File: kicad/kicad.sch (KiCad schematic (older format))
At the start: 40 parts

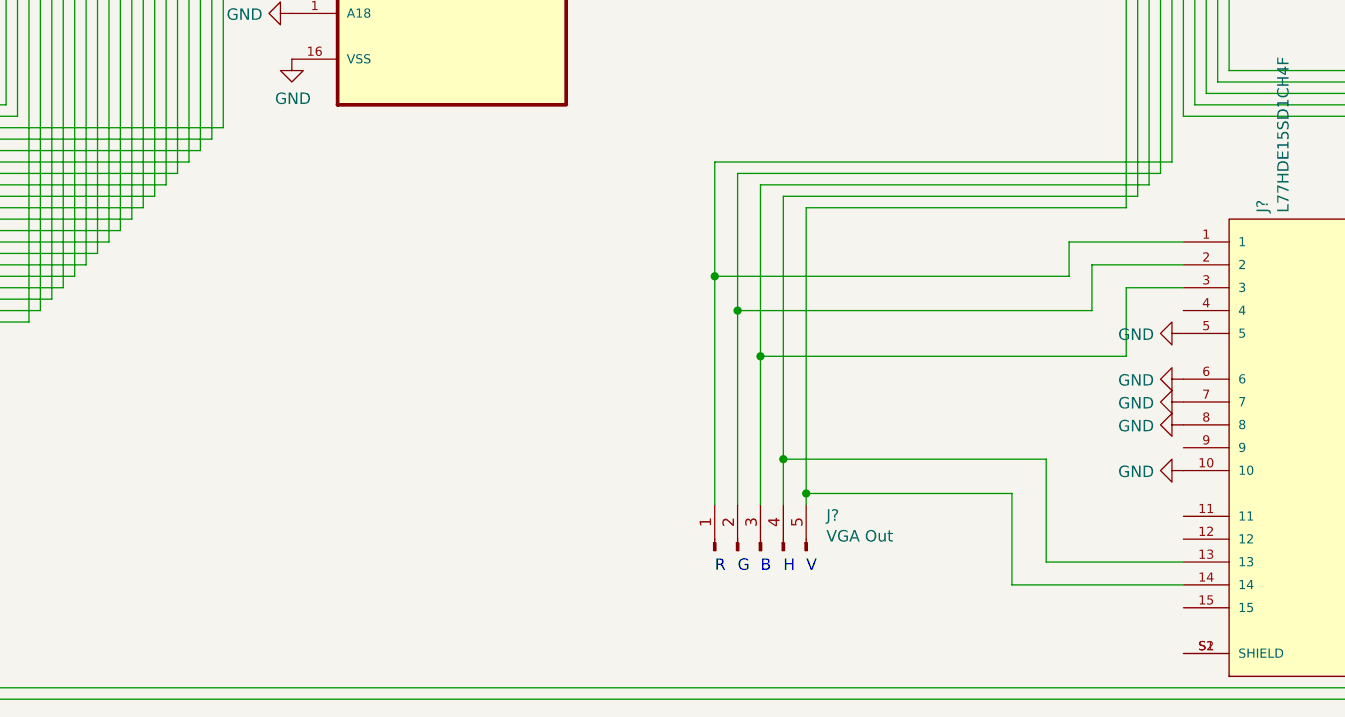
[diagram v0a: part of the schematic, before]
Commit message: Save progress on schematic.
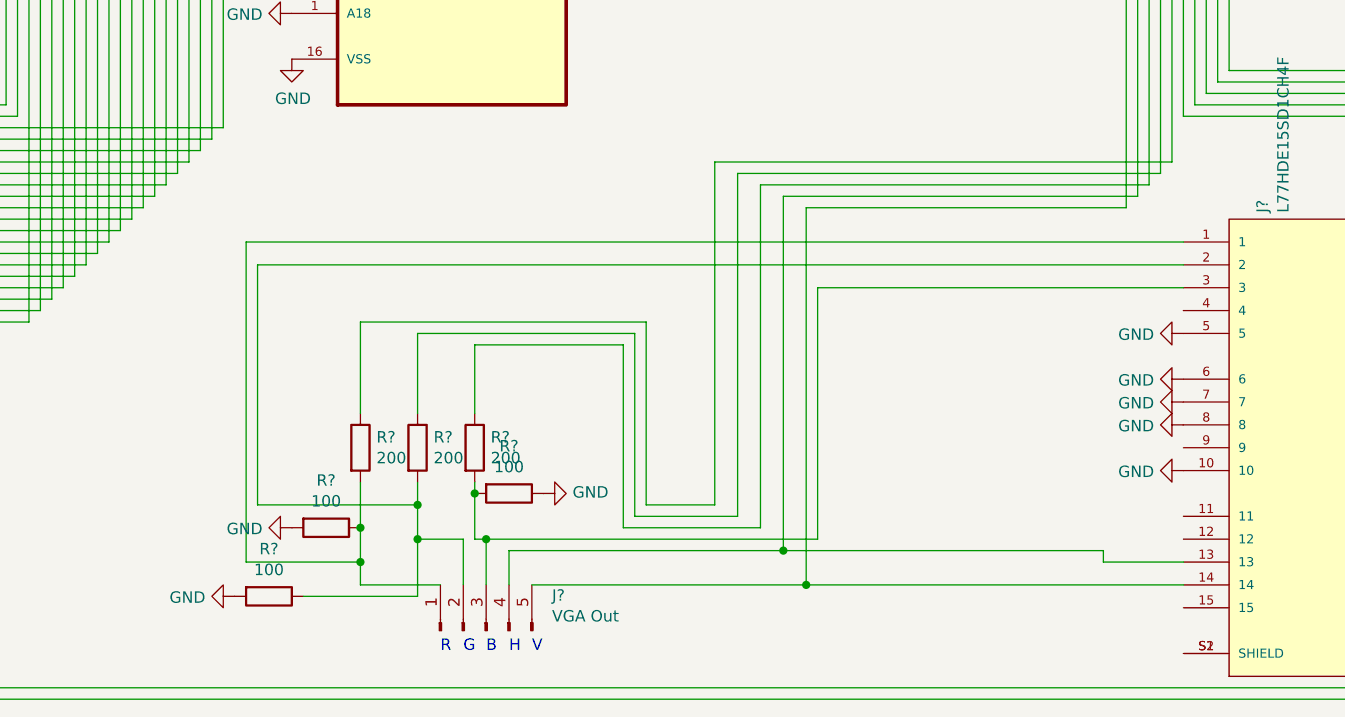
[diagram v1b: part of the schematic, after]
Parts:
- added R? (x3): 200, symbol Device:R
- added R? (x3): 100, symbol Device:R
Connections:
- net GND: now also R?.1, R?.2, R?.2
- net at U?.14 (1Y3), U?.14 (1Y3): now also R?.1; no longer J?.3, J?.3 (Pin_3)
- net at U?.16 (1Y2), U?.16 (1Y2): now also R?.1; no longer J?.2, J?.2 (Pin_2)
- net at U?.18 (1Y1), U?.18 (1Y1): now also R?.1; no longer J?.1, J?.1 (Pin_1)
- new net: J?.1, J?.1 (Pin_1), R?.1, R?.2
- new net: J?.2, J?.2 (Pin_2), R?.1, R?.2
- new net: J?.3, J?.3 (Pin_3), R?.2, R?.2
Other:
- moved on the sheet: J?
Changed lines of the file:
@@
 L Connector:Conn_01x05_Male J?
 U 1 1 634892F6
-P 20900 17550
-F 0 "J?" V 21054 17262 50  0000 R CNN
-F 1 "VGA Out" V 20963 17262 50  0000 R CNN
-F 2 "" H 20900 17550 50  0001 C CNN
-F 3 "~" H 20900 17550 50  0001 C CNN
-	1    20900 17550
+P 19700 17900
+F 0 "J?" V 19854 17612 50  0000 R CNN
+F 1 "VGA Out" V 19763 17612 50  0000 R CNN
+F 2 "" H 19700 17900 50  0001 C CNN
+F 3 "~" H 19700 17900 50  0001 C CNN
+	1    19700 17900
 	0    -1   -1   0
 $EndComp
@@
 	1    0    0    -1
 $EndComp
-Text Notes 20700 17650 0    50   ~ 0
+Text Notes 19500 18000 0    50   ~ 0
 R
-Text Notes 20800 17650 0    50   ~ 0
+Text Notes 19600 18000 0    50   ~ 0
 G
-Text Notes 20900 17650 0    50   ~ 0
+Text Notes 19700 18000 0    50   ~ 0
 B
-Text Notes 21000 17650 0    50   ~ 0
+Text Notes 19800 18000 0    50   ~ 0
 H
-Text Notes 21100 17650 0    50   ~ 0
+Text Notes 19900 18000 0    50   ~ 0
 V
 $Comp
@@
 	22700 15850 20700 15850
 Wire Wire Line
-	20700 15850 20700 16350
-Wire Wire Line
 	22650 13300 22650 15900
 Wire Wire Line
 	22650 15900 20800 15900
 Wire Wire Line
-	20800 15900 20800 16500
-Wire Wire Line
 	22450 13400 22600 13400
 Wire Wire Line
@@
 	22600 15950 20900 15950
 Wire Wire Line
-	20900 15950 20900 16700
-Wire Wire Line
 	22450 13500 22550 13500
 Wire Wire Line
@@
 	22550 16000 21000 16000
 Wire Wire Line
-	21000 16000 21000 17150
-Wire Wire Line
 	22450 13700 22500 13700
 Wire Wire Line
@@
 Wire Wire Line
 	22500 16050 21100 16050
-Wire Wire Line
-	21100 16050 21100 17300
 Wire Wire Line
 	20300 8350 20700 8350
@@
 	20300 8750 20450 8750
 Wire Wire Line
-	20700 16350 22250 16350
-Wire Wire Line
-	22250 16350 22250 16200
-Wire Wire Line
-	22250 16200 22750 16200
-Wire Wire Line
 	1150 18150 25000 18150
-Connection ~ 20700 16350
-Wire Wire Line
-	20700 16350 20700 17350
-Wire Wire Line
-	20800 16500 22350 16500
-Wire Wire Line
-	22350 16500 22350 16300
-Wire Wire Line
-	22350 16300 22750 16300
-Connection ~ 20800 16500
-Wire Wire Line
-	20800 16500 20800 17350
-Wire Wire Line
-	20900 16700 22500 16700
-Wire Wire Line
-	22500 16700 22500 16400
-Wire Wire Line
-	22500 16400 22750 16400
-Connection ~ 20900 16700
-Wire Wire Line
-	20900 16700 20900 17350
-Wire Wire Line
-	21000 17150 22150 17150
-Wire Wire Line
-	22150 17150 22150 17600
-Wire Wire Line
-	22150 17600 22750 17600
-Connection ~ 21000 17150
-Wire Wire Line
-	21000 17150 21000 17350
-Wire Wire Line
-	21100 17300 22000 17300
-Wire Wire Line
-	22000 17300 22000 17700
-Wire Wire Line
-	22000 17700 22750 17700
-Connection ~ 21100 17300
-Wire Wire Line
-	21100 17300 21100 17350
 $Comp
 L power:GND #PWR?
@@
 	0    1    1    0
 $EndComp
+Wire Wire Line
+	20700 15850 20700 17350
+$Comp
+L Device:R R?
+U 1 1 671DFF81
+P 19150 17100
+F 0 "R?" H 19220 17146 50  0000 L CNN
+F 1 "200" H 19220 17055 50  0000 L CNN
+F 2 "" V 19080 17100 50  0001 C CNN
+F 3 "~" H 19150 17100 50  0001 C CNN
+	1    19150 17100
+	1    0    0    -1
+$EndComp
+$Comp
+L Device:R R?
+U 1 1 672CE19D
+P 19400 17100
+F 0 "R?" H 19470 17146 50  0000 L CNN
+F 1 "200" H 19470 17055 50  0000 L CNN
+F 2 "" V 19330 17100 50  0001 C CNN
+F 3 "~" H 19400 17100 50  0001 C CNN
+	1    19400 17100
+	1    0    0    -1
+$EndComp
+$Comp
+L Device:R R?
+U 1 1 672CEC76
+P 19650 17100
+F 0 "R?" H 19720 17146 50  0000 L CNN
+F 1 "200" H 19720 17055 50  0000 L CNN
+F 2 "" V 19580 17100 50  0001 C CNN
+F 3 "~" H 19650 17100 50  0001 C CNN
+	1    19650 17100
+	1    0    0    -1
+$EndComp
+Wire Wire Line
+	19150 17250 19150 17450
+Wire Wire Line
+	19150 17700 19500 17700
+Wire Wire Line
+	19400 17500 19600 17500
+Wire Wire Line
+	19600 17500 19600 17700
+Wire Wire Line
+	19650 17250 19650 17300
+Wire Wire Line
+	19650 17500 19700 17500
+Wire Wire Line
+	19700 17500 19700 17700
+Wire Wire Line
+	20700 17350 20400 17350
+Wire Wire Line
+	20400 17350 20400 16550
+Wire Wire Line
+	20400 16550 19150 16550
+Wire Wire Line
+	19150 16550 19150 16950
+Wire Wire Line
+	20800 17400 20350 17400
+Wire Wire Line
+	20350 17400 20350 16600
+Wire Wire Line
+	20350 16600 19400 16600
+Wire Wire Line
+	19400 16600 19400 16950
+Wire Wire Line
+	20800 15900 20800 17400
+Wire Wire Line
+	20900 17450 20300 17450
+Wire Wire Line
+	20300 17450 20300 16650
+Wire Wire Line
+	20300 16650 19650 16650
+Wire Wire Line
+	19650 16650 19650 16950
+Wire Wire Line
+	20900 15950 20900 17450
+Wire Wire Line
+	21000 17550 19800 17550
+Wire Wire Line
+	19800 17550 19800 17700
+Wire Wire Line
+	21000 16000 21000 17550
+Wire Wire Line
+	21100 17700 19900 17700
+Wire Wire Line
+	21100 16050 21100 17700
+$Comp
+L Device:R R?
+U 1 1 67A61F3B
+P 19000 17450
+F 0 "R?" V 18793 17450 50  0000 C CNN
+F 1 "100" V 18884 17450 50  0000 C CNN
+F 2 "" V 18930 17450 50  0001 C CNN
+F 3 "~" H 19000 17450 50  0001 C CNN
+	1    19000 17450
+	0    1    1    0
+$EndComp
+Connection ~ 19150 17450
+Wire Wire Line
+	19150 17450 19150 17600
+$Comp
+L Device:R R?
+U 1 1 67A62A68
+P 19800 17300
+F 0 "R?" V 19593 17300 50  0000 C CNN
+F 1 "100" V 19684 17300 50  0000 C CNN
+F 2 "" V 19730 17300 50  0001 C CNN
+F 3 "~" H 19800 17300 50  0001 C CNN
+	1    19800 17300
+	0    1    1    0
+$EndComp
+Connection ~ 19650 17300
+Wire Wire Line
+	19650 17300 19650 17500
+$Comp
+L Device:R R?
+U 1 1 67A6355B
+P 18750 17750
+F 0 "R?" V 18543 17750 50  0000 C CNN
+F 1 "100" V 18634 17750 50  0000 C CNN
+F 2 "" V 18680 17750 50  0001 C CNN
+F 3 "~" H 18750 17750 50  0001 C CNN
+	1    18750 17750
+	0    1    1    0
+$EndComp
+Wire Wire Line
+	18900 17750 19400 17750
+Wire Wire Line
+	19400 17250 19400 17350
+Connection ~ 19400 17500
+Wire Wire Line
+	19400 17500 19400 17750
+$Comp
+L power:GND #PWR?
+U 1 1 67B5C404
+P 18850 17450
+F 0 "#PWR?" H 18850 17200 50  0001 C CNN
+F 1 "GND" V 18855 17322 50  0000 R CNN
+F 2 "" H 18850 17450 50  0001 C CNN
+F 3 "" H 18850 17450 50  0001 C CNN
+	1    18850 17450
+	0    1    1    0
+$EndComp
+$Comp
+L power:GND #PWR?
+U 1 1 67B5CCA7
+P 18600 17750
+F 0 "#PWR?" H 18600 17500 50  0001 C CNN
+F 1 "GND" V 18605 17622 50  0000 R CNN
+F 2 "" H 18600 17750 50  0001 C CNN
+F 3 "" H 18600 17750 50  0001 C CNN
+	1    18600 17750
+	0    1    1    0
+$EndComp
+$Comp
+L power:GND #PWR?
+U 1 1 67B5D566
+P 19950 17300
+F 0 "#PWR?" H 19950 17050 50  0001 C CNN
+F 1 "GND" V 19955 17172 50  0000 R CNN
+F 2 "" H 19950 17300 50  0001 C CNN
+F 3 "" H 19950 17300 50  0001 C CNN
+	1    19950 17300
+	0    -1   -1   0
+$EndComp
+Wire Wire Line
+	21000 17550 22400 17550
+Wire Wire Line
+	22400 17550 22400 17600
+Wire Wire Line
+	22400 17600 22750 17600
+Connection ~ 21000 17550
+Wire Wire Line
+	21100 17700 22750 17700
+Connection ~ 21100 17700
+Wire Wire Line
+	19150 17600 18650 17600
+Wire Wire Line
+	18650 17600 18650 16200
+Wire Wire Line
+	18650 16200 22750 16200
+Connection ~ 19150 17600
+Wire Wire Line
+	19150 17600 19150 17700
+Wire Wire Line
+	19400 17350 18700 17350
+Wire Wire Line
+	18700 17350 18700 16300
+Wire Wire Line
+	18700 16300 22750 16300
+Connection ~ 19400 17350
+Wire Wire Line
+	19400 17350 19400 17500
+Wire Wire Line
+	19700 17500 21150 17500
+Wire Wire Line
+	21150 17500 21150 16400
+Wire Wire Line
+	21150 16400 22750 16400
+Connection ~ 19700 17500
 $EndSCHEMATC
